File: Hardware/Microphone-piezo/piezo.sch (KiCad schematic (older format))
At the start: 21 parts, among them J1 RJ14, J2 conn to ground, J3 Conn_01x01_Female, J4 Conn_01x01_Female, J5 Conn_01x01_Female, U1 LME49724, X1 Piezo

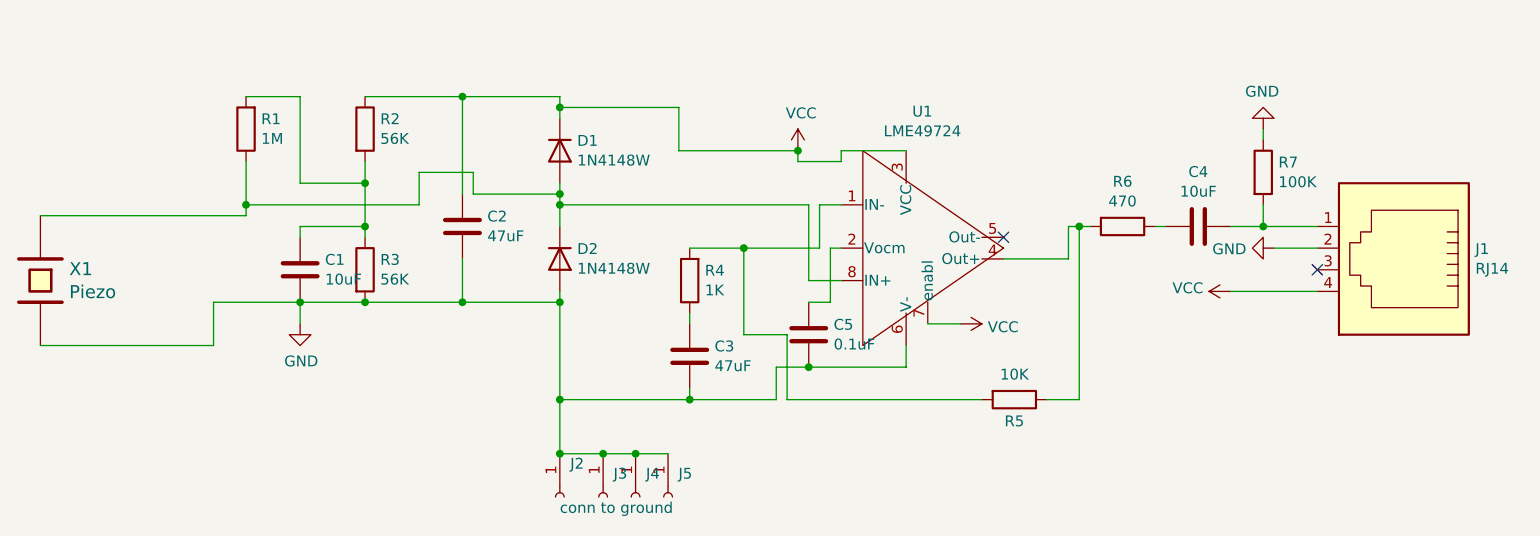
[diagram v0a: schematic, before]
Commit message: Hopefully the final update
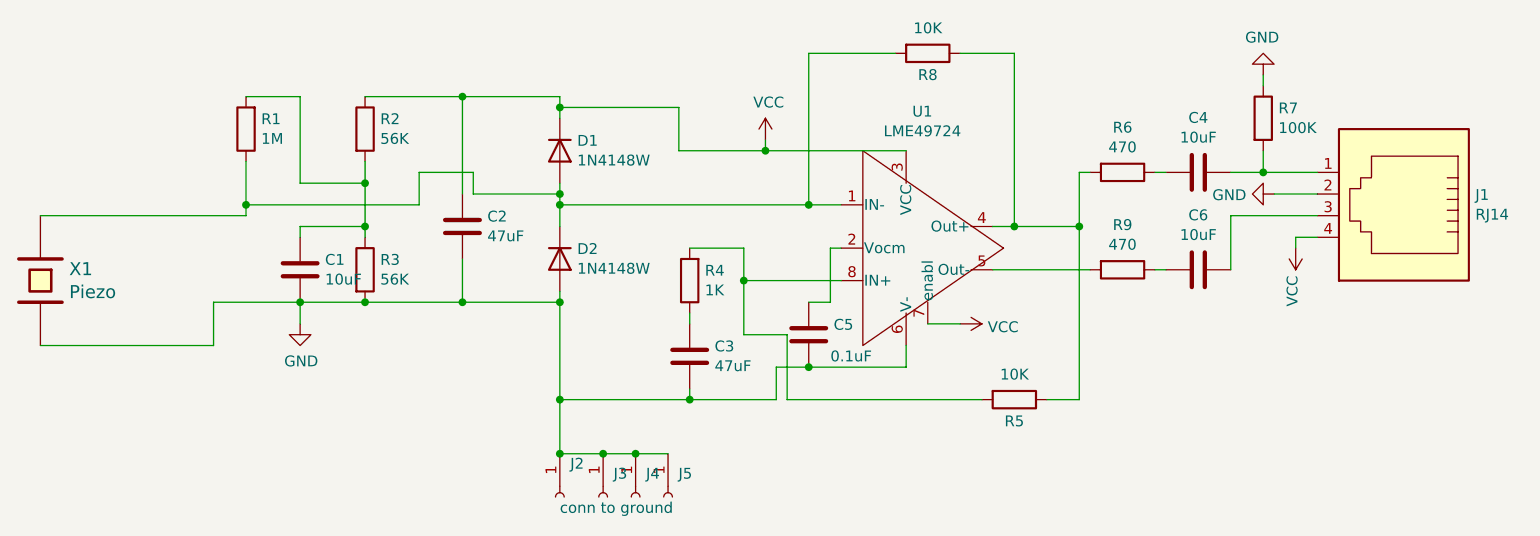
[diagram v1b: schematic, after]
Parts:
- removed U1: LME49724, tastatur:PSOIC-8, symbol keyboard:LME49724
- added C6: 10uF, Capacitor_SMD:CP_Elec_5x5.9, symbol Device:C
- added R8: 10K, Resistor_SMD:R_0603_1608Metric_Pad0.98x0.95mm_HandSolder, symbol Device:R
- added R9: 470, Resistor_SMD:R_0603_1608Metric_Pad0.98x0.95mm_HandSolder, symbol Device:R
- added U1: LME49724, piezo:DDA0008B, symbol Keyboard:LME49724
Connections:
- net GND: now also U1.6 (V-)
- net VCC: now also U1.3 (VCC), U1.7 (enabl)
- net at R5.1, R6.2: now also R8.1, U1.4 (Out+)
- net at R4.2, R5.2: now also U1.8 (IN+)
- net at D1.2 (A), D2.1 (K), R1.1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: now also R8.2, U1.1 (IN-)
- net at J1.3: now also C6.1
- net at C5.1: now also U1.2 (Vocm)
- new net: R9.2, U1.5 (Out-)
- new net: C6.2, R9.1
- no-connect marks 2 -> 0
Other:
- moved on the sheet: C4, J1, R6, R7
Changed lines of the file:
@@
 $EndDescr
 Wire Wire Line
-	7050 4500 6850 4500
+	7050 4250 6850 4250
 $Comp
 L power:GND #PWR05
 U 1 1 5F23E2EA
-P 6850 4500
-F 0 "#PWR05" H 6850 4250 50  0001 C CNN
-F 1 "GND" V 6855 4372 50  0000 R CNN
-F 2 "" H 6850 4500 50  0001 C CNN
-F 3 "" H 6850 4500 50  0001 C CNN
-	1    6850 4500
-	0    1    1    0
-$EndComp
-NoConn ~ 7050 4600
+P 6850 4250
+F 0 "#PWR05" H 6850 4000 50  0001 C CNN
+F 1 "GND" V 6855 4122 50  0000 R CNN
+F 2 "" H 6850 4250 50  0001 C CNN
+F 3 "" H 6850 4250 50  0001 C CNN
+	1    6850 4250
+	0    1    1    0
+$EndComp
 $Comp
 L power:VCC #PWR03
 U 1 1 5F266CDC
-P 6650 4700
-F 0 "#PWR03" H 6650 4550 50  0001 C CNN
-F 1 "VCC" V 6665 4827 50  0000 L CNN
-F 2 "" H 6650 4700 50  0001 C CNN
-F 3 "" H 6650 4700 50  0001 C CNN
-	1    6650 4700
-	0    -1   -1   0
+P 6950 4500
+F 0 "#PWR03" H 6950 4350 50  0001 C CNN
+F 1 "VCC" V 6965 4627 50  0000 L CNN
+F 2 "" H 6950 4500 50  0001 C CNN
+F 3 "" H 6950 4500 50  0001 C CNN
+	1    6950 4500
+	-1   0    0    1
 $EndComp
 $Comp
 L Device:C C4
 U 1 1 5F26F275
-P 6500 4400
-F 0 "C4" V 6248 4400 50  0000 C CNN
-F 1 "10uF" V 6339 4400 50  0000 C CNN
-F 2 "Capacitor_SMD:CP_Elec_5x5.9" H 6538 4250 50  0001 C CNN
-F 3 "~" H 6500 4400 50  0001 C CNN
-	1    6500 4400
-	0    1    1    0
-$EndComp
-Wire Wire Line
-	7050 4700 6650 4700
+P 6500 4150
+F 0 "C4" V 6248 4150 50  0000 C CNN
+F 1 "10uF" V 6339 4150 50  0000 C CNN
+F 2 "Capacitor_SMD:CP_Elec_5x5.9" H 6538 4000 50  0001 C CNN
+F 3 "~" H 6500 4150 50  0001 C CNN
+	1    6500 4150
+	0    1    1    0
+$EndComp
+Wire Wire Line
+	7050 4450 6950 4450
 $Comp
 L Device:R R5
@@
 L Device:R R6
 U 1 1 5F27508E
-P 6150 4400
-F 0 "R6" V 5943 4400 50  0000 C CNN
-F 1 "470" V 6034 4400 50  0000 C CNN
-F 2 "Resistor_SMD:R_0603_1608Metric_Pad1.05x0.95mm_HandSolder" V 6080 4400 50  0001 C CNN
-F 3 "~" H 6150 4400 50  0001 C CNN
-	1    6150 4400
-	0    1    1    0
-$EndComp
-Wire Wire Line
-	6350 4400 6300 4400
-Wire Wire Line
-	6000 4400 5950 4400
-Connection ~ 5950 4400
-Wire Wire Line
-	5950 4400 5900 4400
+P 6150 4150
+F 0 "R6" V 5943 4150 50  0000 C CNN
+F 1 "470" V 6034 4150 50  0000 C CNN
+F 2 "Resistor_SMD:R_0603_1608Metric_Pad1.05x0.95mm_HandSolder" V 6080 4150 50  0001 C CNN
+F 3 "~" H 6150 4150 50  0001 C CNN
+	1    6150 4150
+	0    1    1    0
+$EndComp
+Wire Wire Line
+	6350 4150 6300 4150
+Wire Wire Line
+	6000 4150 5950 4150
 $Comp
 L power:GND #PWR04
 U 1 1 5F286DF2
-P 6800 3950
-F 0 "#PWR04" H 6800 3700 50  0001 C CNN
-F 1 "GND" H 6805 3777 50  0000 C CNN
-F 2 "" H 6800 3950 50  0001 C CNN
-F 3 "" H 6800 3950 50  0001 C CNN
-	1    6800 3950
+P 6800 3700
+F 0 "#PWR04" H 6800 3450 50  0001 C CNN
+F 1 "GND" H 6805 3527 50  0000 C CNN
+F 2 "" H 6800 3700 50  0001 C CNN
+F 3 "" H 6800 3700 50  0001 C CNN
+	1    6800 3700
 	-1   0    0    1
 $EndComp
@@
 L power:VCC #PWR02
 U 1 1 5F2A7038
-P 4650 4050
-F 0 "#PWR02" H 4650 3900 50  0001 C CNN
-F 1 "VCC" H 4665 4223 50  0000 C CNN
-F 2 "" H 4650 4050 50  0001 C CNN
-F 3 "" H 4650 4050 50  0001 C CNN
-	1    4650 4050
-	1    0    0    -1
-$EndComp
-Wire Wire Line
-	4650 4050 4650 4100
+P 4500 4000
+F 0 "#PWR02" H 4500 3850 50  0001 C CNN
+F 1 "VCC" H 4515 4173 50  0000 C CNN
+F 2 "" H 4500 4000 50  0001 C CNN
+F 3 "" H 4500 4000 50  0001 C CNN
+	1    4500 4000
+	1    0    0    -1
+$EndComp
+Wire Wire Line
+	4500 4000 4500 4050
 $Comp
 L Device:D D1
@@
 $EndComp
 Wire Wire Line
-	4400 4900 4400 4500
+	4400 4900 4400 4650
 $Comp
 L Device:C C3
@@
 Wire Wire Line
 	4150 4500 4400 4500
-Connection ~ 4400 4500
 Wire Wire Line
 	2650 4200 2350 4200
@@
 L Device:R R7
 U 1 1 5F2C875E
-P 6800 4150
-F 0 "R7" H 6870 4196 50  0000 L CNN
-F 1 "100K" H 6870 4105 50  0000 L CNN
-F 2 "Resistor_SMD:R_0603_1608Metric_Pad1.05x0.95mm_HandSolder" V 6730 4150 50  0001 C CNN
-F 3 "~" H 6800 4150 50  0001 C CNN
-	1    6800 4150
-	1    0    0    -1
-$EndComp
-Wire Wire Line
-	7050 4400 6800 4400
-Wire Wire Line
-	6800 4300 6800 4400
-Connection ~ 6800 4400
-Wire Wire Line
-	6800 4400 6650 4400
-Wire Wire Line
-	6800 4000 6800 3950
+P 6800 3900
+F 0 "R7" H 6870 3946 50  0000 L CNN
+F 1 "100K" H 6870 3855 50  0000 L CNN
+F 2 "Resistor_SMD:R_0603_1608Metric_Pad1.05x0.95mm_HandSolder" V 6730 3900 50  0001 C CNN
+F 3 "~" H 6800 3900 50  0001 C CNN
+	1    6800 3900
+	1    0    0    -1
+$EndComp
+Wire Wire Line
+	7050 4150 6800 4150
+Wire Wire Line
+	6800 4050 6800 4150
+Connection ~ 6800 4150
+Wire Wire Line
+	6800 4150 6650 4150
+Wire Wire Line
+	6800 3750 6800 3700
 Wire Wire Line
 	2650 3800 3100 3800
@@
 	3550 3800 3550 3850
 Wire Wire Line
-	4650 4050 4100 4050
-Wire Wire Line
-	4100 4050 4100 3850
-Wire Wire Line
 	4100 3850 3550 3850
-Connection ~ 4650 4050
 Connection ~ 3550 3850
 Wire Wire Line
@@
 L Connector:RJ14 J1
 U 1 1 5F2F3AAF
-P 7450 4500
-F 0 "J1" H 7120 4504 50  0000 R CNN
-F 1 "RJ14" H 7120 4595 50  0000 R CNN
-F 2 "Connector_RJ:RJ14_Connfly_DS1133-S4_Horizontal" V 7450 4525 50  0001 C CNN
-F 3 "~" V 7450 4525 50  0001 C CNN
-	1    7450 4500
+P 7450 4250
+F 0 "J1" H 7120 4254 50  0000 R CNN
+F 1 "RJ14" H 7120 4345 50  0000 R CNN
+F 2 "Connector_RJ:RJ14_Connfly_DS1133-S4_Horizontal" V 7450 4275 50  0001 C CNN
+F 3 "~" V 7450 4275 50  0001 C CNN
+	1    7450 4250
 	-1   0    0    1
 $EndComp
@@
 Wire Wire Line
 	2100 4300 2100 4350
-$Comp
-L keyboard:LME49724 U1
-U 1 1 607482EC
-P 5350 4500
-F 0 "U1" H 5225 5131 50  0000 C CNN
-F 1 "LME49724" H 5225 5040 50  0000 C CNN
-F 2 "tastatur:PSOIC-8" H 5100 3800 50  0001 C CIN
-F 3 "http://www.ti.com/lit/ds/symlink/lme49600.pdf" H 5350 4500 50  0001 C CNN
-	1    5350 4500
-	1    0    0    -1
-$EndComp
-Wire Wire Line
-	4850 4650 4700 4650
-Wire Wire Line
-	4700 4650 4700 4300
-Wire Wire Line
-	3550 4300 4700 4300
-Wire Wire Line
-	4750 4500 4750 4300
-Wire Wire Line
-	4750 4300 4850 4300
-Wire Wire Line
-	4400 4500 4750 4500
-Wire Wire Line
-	4650 4100 4850 4100
-Wire Wire Line
-	4850 4100 4850 4050
-Wire Wire Line
-	4850 4050 5150 4050
 Wire Wire Line
 	4550 5200 4550 5050
@@
 P 4700 4900
 F 0 "C5" H 4815 4946 50  0000 L CNN
-F 1 "0.1uF" H 4815 4855 50  0000 L CNN
+F 1 "0.1uF" H 4800 4800 50  0000 L CNN
 F 2 "Capacitor_SMD:CP_Elec_5x5.9" H 4738 4750 50  0001 C CNN
 F 3 "~" H 4700 4900 50  0001 C CNN
@@
 Wire Wire Line
 	4800 4500 4850 4500
-Wire Wire Line
-	5600 4550 5900 4550
-Wire Wire Line
-	5900 4550 5900 4400
-NoConn ~ 5600 4450
 $Comp
 L power:VCC #PWR0101
@@
 Wire Wire Line
 	4700 5050 5150 5050
+$Comp
+L Keyboard:LME49724 U1
+U 1 1 6075AE2F
+P 5350 4500
+F 0 "U1" H 5225 5131 50  0000 C CNN
+F 1 "LME49724" H 5225 5040 50  0000 C CNN
+F 2 "piezo:DDA0008B" H 5100 3800 50  0001 C CIN
+F 3 "http://www.ti.com/lit/ds/symlink/lme49600.pdf" H 5350 4500 50  0001 C CNN
+	1    5350 4500
+	1    0    0    -1
+$EndComp
+Wire Wire Line
+	5550 4400 5650 4400
+Wire Wire Line
+	5950 4400 5950 4150
+Connection ~ 5950 4400
+Wire Wire Line
+	6950 4500 6950 4450
+$Comp
+L Device:R R9
+U 1 1 60779FC0
+P 6150 4600
+F 0 "R9" V 5943 4600 50  0000 C CNN
+F 1 "470" V 6034 4600 50  0000 C CNN
+F 2 "Resistor_SMD:R_0603_1608Metric_Pad0.98x0.95mm_HandSolder" V 6080 4600 50  0001 C CNN
+F 3 "~" H 6150 4600 50  0001 C CNN
+	1    6150 4600
+	0    1    1    0
+$EndComp
+$Comp
+L Device:C C6
+U 1 1 6077AA47
+P 6500 4600
+F 0 "C6" V 6248 4600 50  0000 C CNN
+F 1 "10uF" V 6339 4600 50  0000 C CNN
+F 2 "Capacitor_SMD:CP_Elec_5x5.9" H 6538 4450 50  0001 C CNN
+F 3 "~" H 6500 4600 50  0001 C CNN
+	1    6500 4600
+	0    1    1    0
+$EndComp
+Wire Wire Line
+	7050 4350 6650 4350
+Wire Wire Line
+	6650 4350 6650 4600
+Wire Wire Line
+	6350 4600 6300 4600
+Wire Wire Line
+	6000 4600 5550 4600
+$Comp
+L Device:R R8
+U 1 1 60781143
+P 5250 3600
+F 0 "R8" V 5350 3600 50  0000 C CNN
+F 1 "10K" V 5134 3600 50  0000 C CNN
+F 2 "Resistor_SMD:R_0603_1608Metric_Pad0.98x0.95mm_HandSolder" V 5180 3600 50  0001 C CNN
+F 3 "~" H 5250 3600 50  0001 C CNN
+	1    5250 3600
+	0    1    1    0
+$EndComp
+Wire Wire Line
+	5650 4400 5650 3600
+Wire Wire Line
+	5650 3600 5400 3600
+Connection ~ 5650 4400
+Wire Wire Line
+	5650 4400 5950 4400
+Wire Wire Line
+	3550 4300 4700 4300
+Wire Wire Line
+	4500 4050 4100 4050
+Wire Wire Line
+	4100 4050 4100 3850
+Connection ~ 4500 4050
+Wire Wire Line
+	4500 4050 5150 4050
+Wire Wire Line
+	5100 3600 4700 3600
+Wire Wire Line
+	4700 3600 4700 4300
+Wire Wire Line
+	4700 4300 4850 4300
+Connection ~ 4700 4300
+Wire Wire Line
+	4850 4650 4400 4650
+Connection ~ 4400 4650
+Wire Wire Line
+	4400 4650 4400 4500
 $EndSCHEMATC
